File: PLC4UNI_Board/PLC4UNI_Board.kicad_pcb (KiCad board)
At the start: 2 copper layers, 104.2 x 84.9 mm, 16 parts, among them J1 NPN_OUT, J10 RLY_OUT, J11 RLY2_OUT, J12 0-10_AC, J2 NPN_IN, J3 AN_IN_OUT, J4 ANA_V_0-10, J5 CT_TC, J6 RS_485, J7 PNP_OUT, J8 24_V_DC, J9 PNP_IN, U1 ESP32-S3-WR-1, U2 AP63203WU

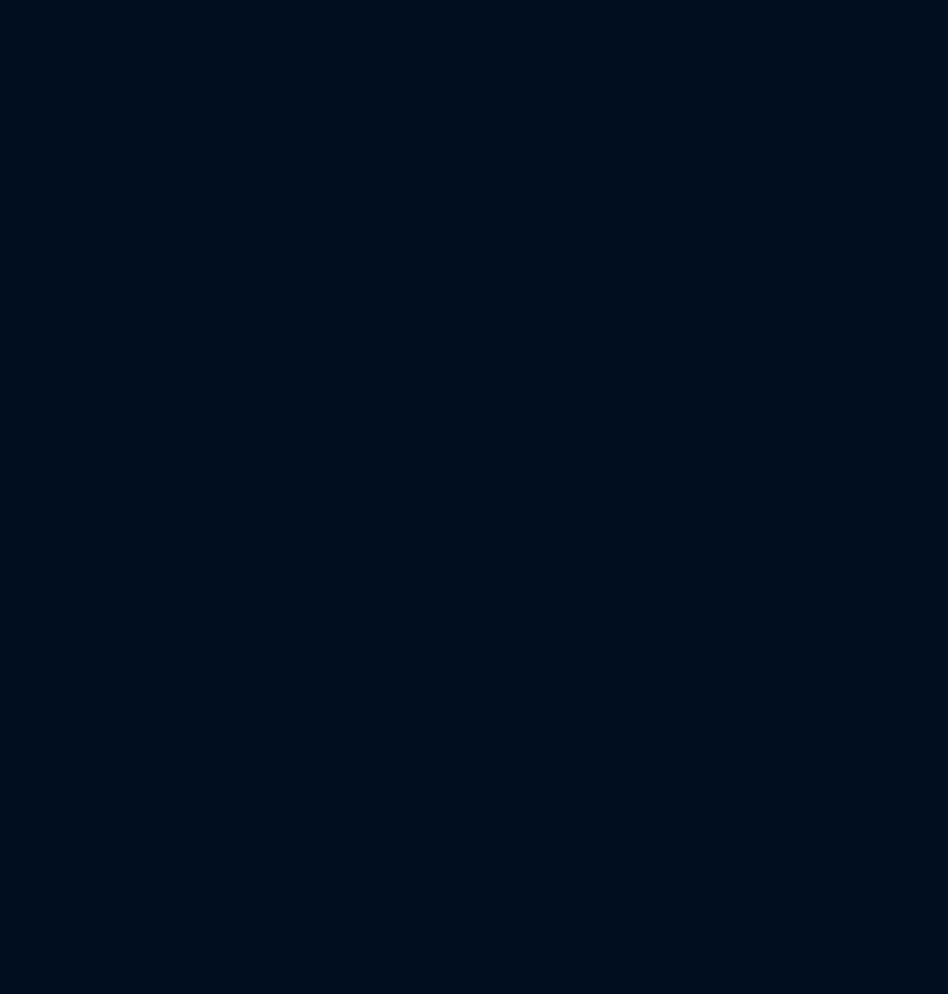
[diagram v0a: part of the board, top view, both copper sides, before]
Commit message: V1.0.2 PLC4UNI
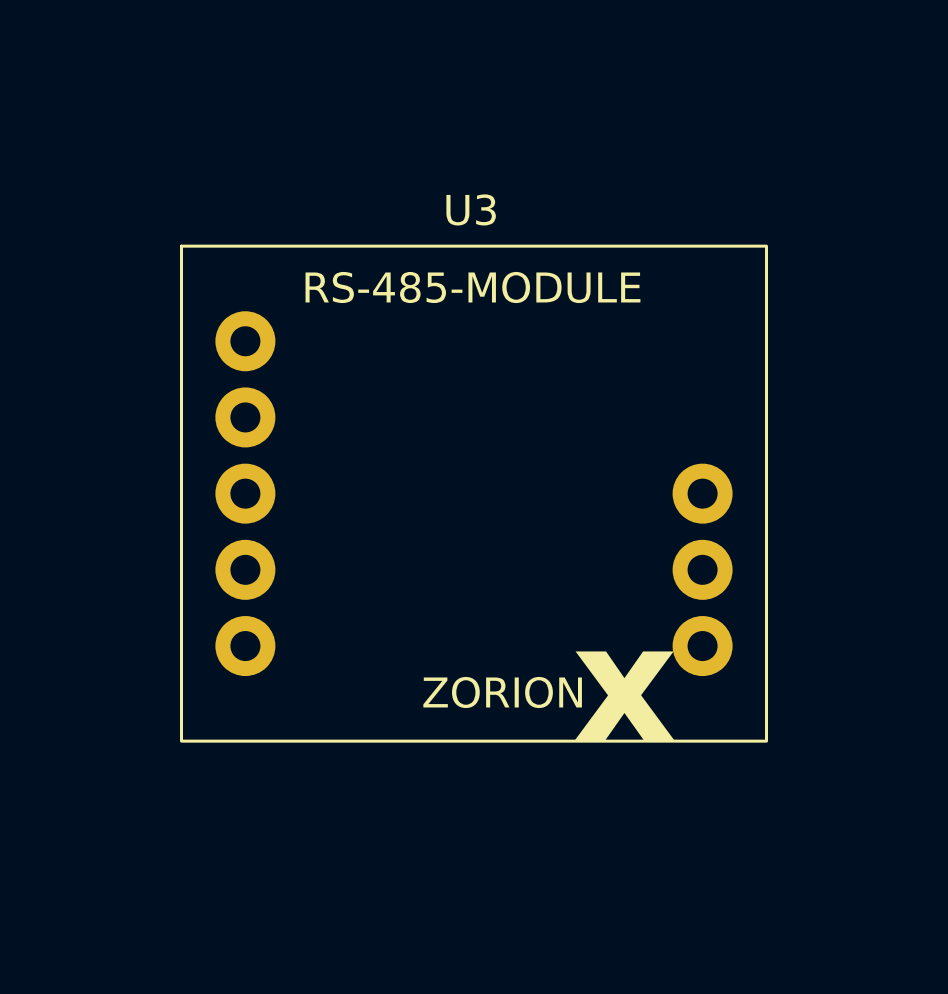
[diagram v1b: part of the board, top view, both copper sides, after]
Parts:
- added U3: ~, sarihuella:RS485-MODULE-DEVO, F.Cu at (230.6, 106.2)
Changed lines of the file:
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@@
 		)
+	)
+	(footprint "sarihuella:RS485-MODULE-DEVO"
+		(layer "F.Cu")
+		(at 230.63 106.25)
+		(property "Reference" "U3"
+			(at 9.65 -17.67 0)
+			(unlocked yes)
+			(layer "F.SilkS")
+			(effects
+				(font
+					(size 1 1)
+					(thickness 0.1)
+				)
+			)
+		)
+		(property "Value" "~"
+			(at 6.87 -19.17 0)
+			(unlocked yes)
+			(layer "F.Fab")
+			(effects
+				(font
+					(size 1 1)
+					(thickness 0.15)
+				)
+			)
+		)
+		(property "Datasheet" ""
+			(at 0 0 0)
+			(unlocked yes)
+			(layer "F.Fab")
+			(hide yes)
+			(effects
+				(font
+					(size 1 1)
+					(thickness 0.15)
+				)
+			)
+		)
+		(property "Description" ""
+			(at 0 0 0)
+			(unlocked yes)
+			(layer "F.Fab")
+			(hide yes)
+			(effects
+				(font
+					(size 1 1)
+					(thickness 0.15)
+				)
+			)
+		)
+		(sheetname "/PLC4UNI/RS485/")
+		(sheetfile "RS485.kicad_sch")
+		(attr smd)
+		(fp_rect
+			(start 0 -16.5)
+			(end 19.5 0)
+			(stroke
+				(width 0.1)
+				(type solid)
+			)
+			(fill no)
+			(layer "F.SilkS")
+		)
+		(fp_text user "x"
+			(at 13 0.5 0)
+			(unlocked yes)
+			(layer "F.SilkS")
+			(effects
+				(font
+					(face "Britannic Bold")
+					(size 4 4)
+					(thickness 0.2)
+					(bold yes)
+				)
+				(justify left bottom)
+			)
+			(render_cache "x" 0
+				(polygon
+					(pts
+						(xy 246.202609 103.303217) (xy 245.384884 104.411346) (xy 246.320823 106.07) (xy 245.160669 106.07)
+						(xy 244.648004 105.175582) (xy 243.988792 106.07) (xy 243.587013 106.07) (xy 244.475568 104.866371)
+						(xy 243.597027 103.303217) (xy 244.762798 103.303217) (xy 245.210006 104.096273) (xy 245.80083 103.303217)
+					)
+				)
+			)
+		)
+		(fp_text user "RS-485-MODULE"
+			(at 4 -14.5 0)
+			(unlocked yes)
+			(layer "F.SilkS")
+			(effects
+				(font
+					(size 1 1)
+					(thickness 0.1)
+				)
+				(justify left bottom)
+			)
+		)
+		(fp_text user "ZORION"
+			(at 8 -1 0)
+			(unlocked yes)
+			(layer "F.SilkS")
+			(effects
+				(font
+					(size 1 1)
+					(thickness 0.1)
+				)
+				(justify left bottom)
+			)
+		)
+		(fp_text user "RS485"
+			(at 10.37 -19.17 0)
+			(unlocked yes)
+			(layer "F.Fab")
+			(effects
+				(font
+					(size 1 1)
+					(thickness 0.15)
+				)
+			)
+		)
+		(pad "1" thru_hole circle
+			(at 2.13 -3.17)
+			(size 2 2)
+			(drill 1)
+			(layers "*.Cu" "*.Mask")
+			(remove_unused_layers no)
+		)
+		(pad "1" thru_hole circle
+			(at 17.37 -8.25)
+			(size 2 2)
+			(drill 1)
+			(layers "*.Cu" "*.Mask")
+			(remove_unused_layers no)
+		)
+		(pad "2" thru_hole circle
+			(at 2.13 -5.71)
+			(size 2 2)
+			(drill 1)
+			(layers "*.Cu" "*.Mask")
+			(remove_unused_layers no)
+		)
+		(pad "2" thru_hole circle
+			(at 17.37 -5.71)
+			(size 2 2)
+			(drill 1)
+			(layers "*.Cu" "*.Mask")
+			(remove_unused_layers no)
+		)
+		(pad "3" thru_hole circle
+			(at 2.13 -8.25)
+			(size 2 2)
+			(drill 1)
+			(layers "*.Cu" "*.Mask")
+			(remove_unused_layers no)
+		)
+		(pad "3" thru_hole circle
+			(at 17.37 -3.17)
+			(size 2 2)
+			(drill 1)
+			(layers "*.Cu" "*.Mask")
+			(remove_unused_layers no)
+		)
+		(pad "4" thru_hole circle
+			(at 2.13 -10.79)
+			(size 2 2)
+			(drill 1)
+			(layers "*.Cu" "*.Mask")
+			(remove_unused_layers no)
+		)
+		(pad "5" thru_hole circle
+			(at 2.13 -13.33)
+			(size 2 2)
+			(drill 1)
+			(layers "*.Cu" "*.Mask")
+			(remove_unused_layers no)
+		)
+		(embedded_fonts no)
 	)
 	(footprint "tb-003H:EBBA-02-C-SS-BU"

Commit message: main
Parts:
- removed J1: NPN_OUT, tb-002H:TE_796683-4
- removed J10: RLY_OUT, TB'000H:tb
- removed J11: RLY2_OUT, tb-003H:EBBA-02-C-SS-BU
- removed J12: 0-10_AC, tb-003H:EBBA-02-C-SS-BU
- removed J2: NPN_IN, tb-002H:TE_796683-4
- removed J3: AN_IN_OUT, TB'000H:terminal block
- removed J4: ANA_V_0-10, tb-003H:EBBA-02-C-SS-BU
- removed J5: CT_TC, tb-003H:EBBA-02-C-SS-BU
- removed J6: RS_485, TB'000H:tb
- removed J7: PNP_OUT, TB'000H:terminal block
- removed J8: 24_V_DC, tb-003H:EBBA-02-C-SS-BU
- removed J9: PNP_IN, tb-002H:TE_796683-4
- removed L2: 6.8uH_1.0A_4018, Inductor_SMD:L_APV_ANR6028
- removed TR1: ZMCT103C, Transformer_THT:Transformer_Zeming_ZMCT103C
- removed U1: ESP32-S3-WR-1, RF_Module:ESP32-S3-WROOM-1
- removed U2: AP63203WU, Package_TO_SOT_SMD:TSOT-23-6
- removed U3: ~, sarihuella:RS485-MODULE-DEVO

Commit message: v.1.0.1
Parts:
- added J1: NPN_OUT, tb-002H:TE_796683-4, F.Cu at (226.0, 60.0)
- added J10: RLY_OUT, TB'000H:tb, F.Cu at (278.0, 134.8)
- added J11: RLY2_OUT, tb-003H:EBBA-02-C-SS-BU, F.Cu at (290.5, 135.5)
- added J12: 0-10_AC, tb-003H:EBBA-02-C-SS-BU, F.Cu at (291.0, 60.5)
- added J2: NPN_IN, tb-002H:TE_796683-4, F.Cu at (247.0, 60.0)
- added J3: AN_IN_OUT, TB'000H:terminal block, F.Cu at (205.0, 60.0)
- added J4: ANA_V_0-10, tb-003H:EBBA-02-C-SS-BU, F.Cu at (270.5, 60.5)
- added J5: CT_TC, tb-003H:EBBA-02-C-SS-BU, F.Cu at (281.0, 60.5)
- added J6: RS_485, TB'000H:tb, F.Cu at (221.0, 134.8)
- added J7: PNP_OUT, TB'000H:terminal block, F.Cu at (231.0, 135.0)
- added J8: 24_V_DC, tb-003H:EBBA-02-C-SS-BU, F.Cu at (208.0, 135.5)
- added J9: PNP_IN, tb-002H:TE_796683-4, F.Cu at (252.0, 135.0)
- added L2: 6.8uH_1.0A_4018, Inductor_SMD:L_APV_ANR6028, F.Cu at (74.2, 91.4)
- added TR1: ZMCT103C, Transformer_THT:Transformer_Zeming_ZMCT103C, F.Cu at (74.5, 79.7)
- added U1: ESP32-S3-WR-1, RF_Module:ESP32-S3-WROOM-1, F.Cu at (43.8, 101.9)
- added U2: AP63203WU, Package_TO_SOT_SMD:TSOT-23-6, F.Cu at (72.9, 97.5)
